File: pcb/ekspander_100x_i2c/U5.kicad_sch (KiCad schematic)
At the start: 12 parts, among them J12 DG127A-5.08-06P-14-00AH, J13 DG127A-5.08-06P-14-00AH, J14 DG127A-5.08-06P-14-00AH, U26 LTV-847, U27 ITS716G, U28 ITS716G, U29 LTV-847, U5 MCP23017_SP

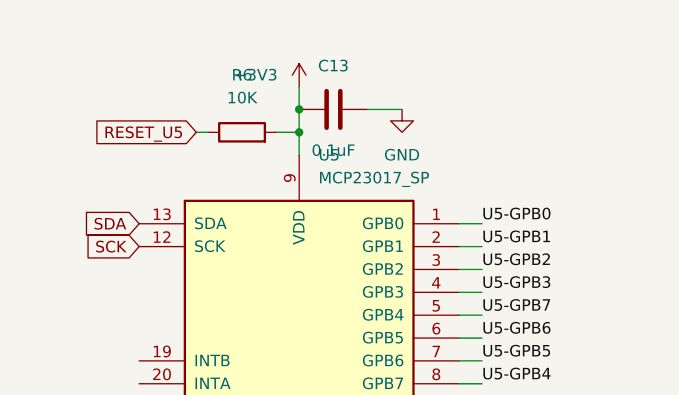
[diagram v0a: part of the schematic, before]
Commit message: Tech Explorations
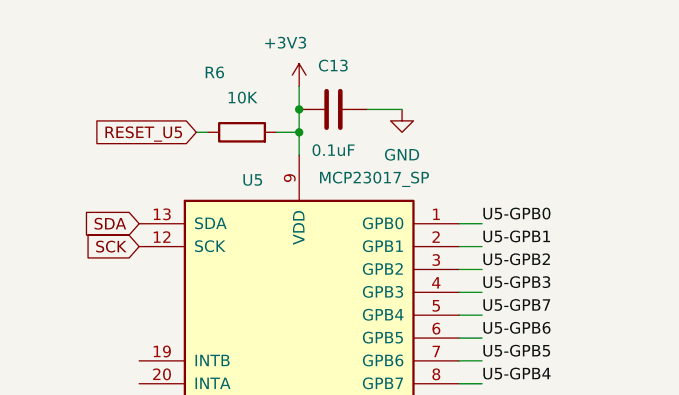
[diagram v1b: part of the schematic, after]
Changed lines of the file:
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@@
 		)
 		(property "Value" "+3V3"
-			(at 44.704 21.59 0)
+			(at 48.006 18.034 0)
 			(effects
 				(font
@@
 		(on_board yes)
 		(dnp no)
-		(fields_autoplaced yes)
 		(property "Reference" "R6"
-			(at 43.18 21.59 90)
+			(at 40.132 21.336 90)
 			(effects
 				(font
@@
 		(on_board yes)
 		(dnp no)
-		(fields_autoplaced yes)
 		(property "Reference" "U5"
-			(at 51.6733 30.48 0)
-			(effects
-				(font
+			(at 43.18 33.274 0)
+			(effects
+				(font
